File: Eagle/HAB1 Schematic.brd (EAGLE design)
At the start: 68.2 x 55.9 mm, 17 parts, among them U1 microSD

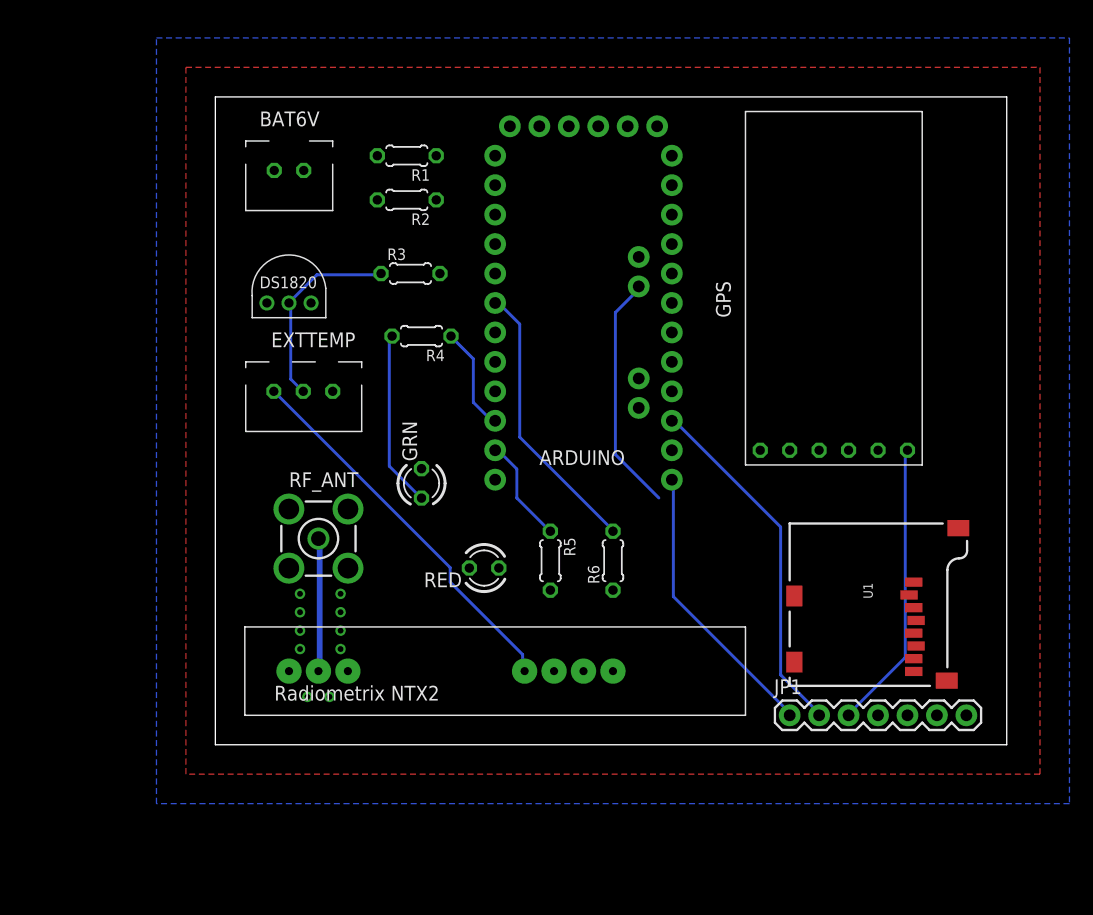
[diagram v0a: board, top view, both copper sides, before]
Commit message: Update
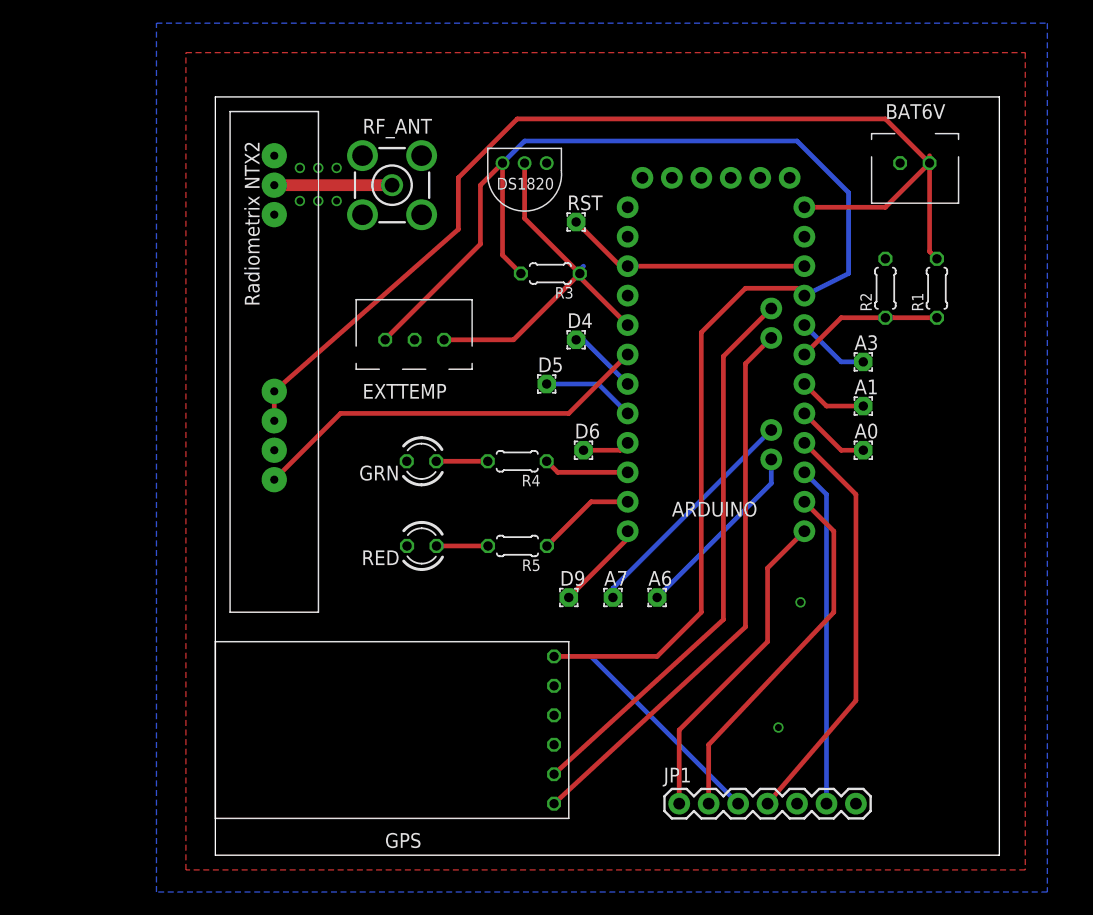
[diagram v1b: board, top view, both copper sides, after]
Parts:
- removed R6: 10K, rcl:0204/5
- removed U1: microSD, SparkFun:MICRO-SD-SOCKET-PP
- added A0: A0, wirepad:1,6/0,8
- added A1: A1, wirepad:1,6/0,8
- added A3: A3, wirepad:1,6/0,8
- added A6: A6, wirepad:1,6/0,8
- added A7: A7, wirepad:1,6/0,8
- added D4: D4, wirepad:1,6/0,8
- added D5: D5, wirepad:1,6/0,8
- added D6: D6, wirepad:1,6/0,8
- added D9: D9, wirepad:1,6/0,8
- added RST: RST, wirepad:1,6/0,8
- GRN, RED: value (none) -> LED
- JP1: value (none) -> SD
- moved BAT6V 54.0 mm to (61.6, 66.7)
- moved R1 47.1 mm to (62.2, 53.3), turned to 90 degrees
- moved GPS 46.7 mm to (20.3, 14.0), turned to 90 degrees
- moved R2 42.0 mm to (57.8, 53.3), turned to 90 degrees
- moved U$3 37.9 mm to (5.08, 57.1), turned to 270 degrees
- moved RF_ANT 31.1 mm to (15.2, 62.2)
- moved INT 27.1 mm to (29.2, 62.9), turned to 180 degrees
- moved R4 13.6 mm to (26.0, 38.4)
- moved ARDUINO 12.3 mm to (43.2, 47.6)
- moved JP1 12.2 mm to (40.0, 8.89)
- moved R3 12.1 mm to (28.9, 54.6), turned to 180 degrees
- moved EXTTEMP 9.55 mm to (17.1, 46.4), turned to 180 degrees
- moved RED 5.70 mm to (17.8, 31.1)
- moved R5 3.11 mm to (26.1, 31.1), turned to 180 degrees
- moved GRN 1.90 mm to (17.8, 38.4), turned to 180 degrees
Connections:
- net CS renamed N$1
- net SCK renamed N$21
- removed net DI: ARDUINO.15, JP1.2
- removed net DO: ARDUINO.14, JP1.6
- removed net N$1 (its old number): R6.1, U$3.TXD
- new net A0: A0.1, ARDUINO.17
- new net A1: A1.1, ARDUINO.18
- new net A3: A3.1, ARDUINO.20
- new net A6: A6.1, ARDUINO.A6
- new net A7: A7.1, ARDUINO.A7
- new net D4: ARDUINO.7, D4.1
- new net D5: ARDUINO.8, D5.1
- new net D6: ARDUINO.9, D6.1
- new net D9: ARDUINO.12, D9.1
- new net N$19: ARDUINO.15, JP1.6
- new net N$20: ARDUINO.14, JP1.2
- new net RST: ARDUINO.22, ARDUINO.3, RST.1
- net GND: now also ARDUINO.4
- net N$6: now also U$3.TXD; no longer R6.2
- net RAW: now also U$3.EN, U$3.VCC
- net VCC: no longer U$3.EN, U$3.VCC
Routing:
- net RAW: track 0.00 -> 94.0 mm
- net VCC: track 58.1 -> 143.6 mm
- net N$8: track 0.00 -> 48.3 mm
- net N$21: track 0.00 -> 35.8 mm
- net N$20: track 0.00 -> 31.4 mm
- net DI: track 30.8 -> 0.00 mm
- net N$19: track 0.00 -> 29.4 mm
- net N$50: track 20.6 -> 48.3 mm
- net RST: track 0.00 -> 21.3 mm
- net A7: track 0.00 -> 20.1 mm
- net A6: track 0.00 -> 16.0 mm
- net D2: track 17.2 -> 32.8 mm
- net A2: track 0.00 -> 12.7 mm
- net N$3: track 15.2 -> 4.45 mm
- net N$6: track 24.2 -> 35.0 mm
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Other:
- board size 68.2 x 55.9 mm -> 67.6 x 65.4 mm
- board text removed: "OK"
- board text removed: "WARN"

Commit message: Updated PCB
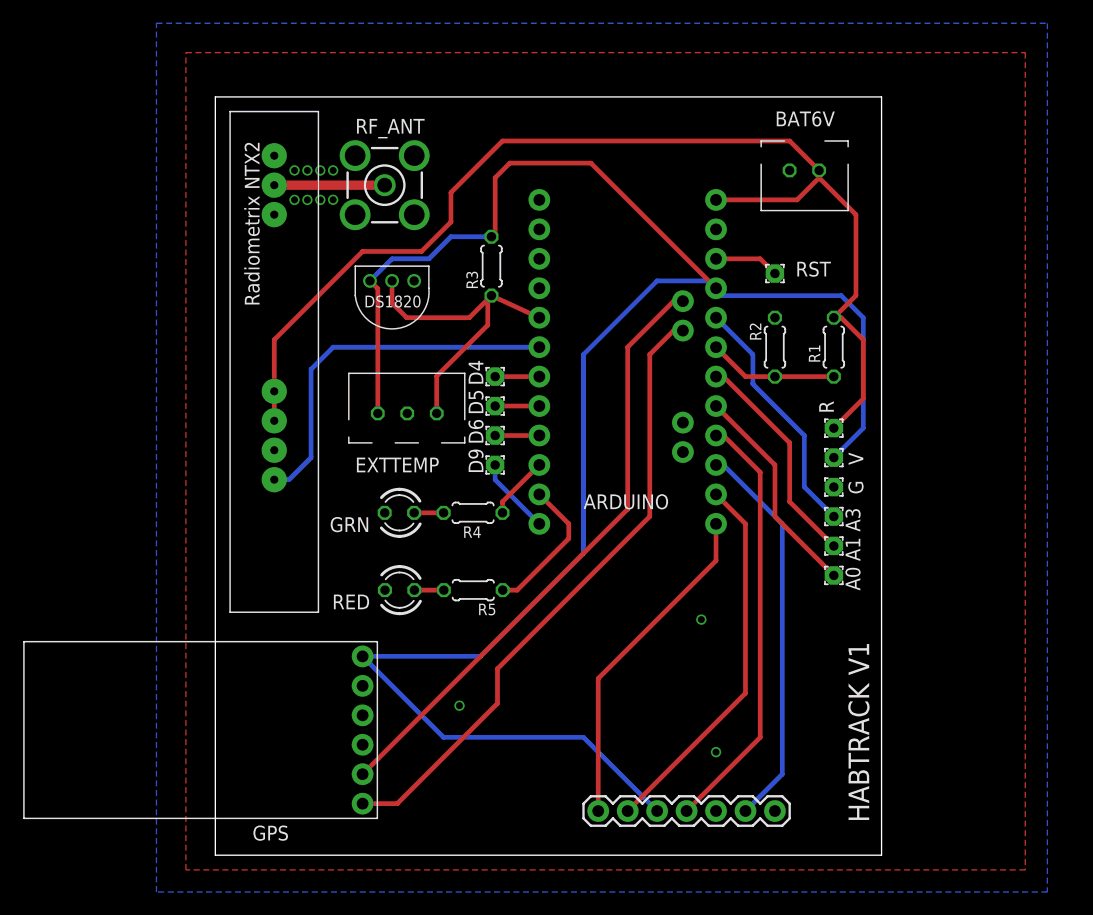
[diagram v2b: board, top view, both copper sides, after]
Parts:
- removed A6: A6, wirepad:1,6/0,8
- removed A7: A7, wirepad:1,6/0,8
- added GND: GND, wirepad:1,6/0,8
- added RAW: RAW, wirepad:1,6/0,8
- added VCC: VCC, wirepad:1,6/0,8
- R1: value 100 -> 10K
- R2: value 50 -> 4K7
- moved RST 17.7 mm to (48.3, 54.6)
- moved GPS 16.5 mm to (3.81, 14.0)
- moved INT 15.3 mm to (17.8, 52.7)
- moved A3 13.6 mm to (53.3, 33.7), turned to 270 degrees
- moved D9 13.1 mm to (24.1, 38.1), turned to 90 degrees
- moved A1 12.3 mm to (53.3, 31.1), turned to 270 degrees
- moved A0 11.1 mm to (53.3, 28.6), turned to 270 degrees
- moved R2 10.8 mm to (48.3, 48.3)
- moved R1 10.2 mm to (53.3, 48.3)
- moved BAT6V 9.55 mm to (52.1, 66.0)
- moved D6 7.73 mm to (24.1, 40.6), turned to 90 degrees
- moved D4 7.67 mm to (24.1, 45.7), turned to 90 degrees
- moved ARDUINO 7.65 mm to (35.6, 48.3)
- moved JP1 7.01 mm to (33.0, 8.26)
- moved EXTTEMP 6.38 mm to (16.5, 40.0)
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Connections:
- removed net A6: A6.1, ARDUINO.A6
- removed net A7: A7.1, ARDUINO.A7
- net GND: now also GND.1
- net RAW: now also RAW.1
- net RST: no longer ARDUINO.3
- net VCC: now also VCC.1
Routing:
- net VCC: track 143.6 -> 164.8 mm
- net A7: track 20.1 -> 0.00 mm
- net A6: track 16.0 -> 0.00 mm
- net RST: track 21.3 -> 5.61 mm
- net A3: track 6.40 -> 21.4 mm
- net A1: track 5.87 -> 19.2 mm
- net A0: track 6.40 -> 18.8 mm
- net N$50: track 48.3 -> 54.5 mm
- net RAW: track 94.0 -> 100.1 mm
- net N$19: track 29.4 -> 33.9 mm
- net N$8: track 48.3 -> 52.7 mm
- net D2: track 32.8 -> 28.5 mm
- net D5: track 8.04 -> 3.81 mm
- net N$4: track 8.54 -> 12.4 mm
- net N$6: track 35.0 -> 32.1 mm
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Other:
- board size 67.6 x 65.4 mm -> 57.5 x 65.4 mm
- board text added: "G"
- board text added: "R"
- board text added: "V"
- board text added: "XxXxXxXxXxXx"
